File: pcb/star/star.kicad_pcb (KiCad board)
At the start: 2 copper layers, 58.9 x 56 mm, 24 parts, among them J1 POWER, U1 ESP-12F, U2 AP2112K-3.3

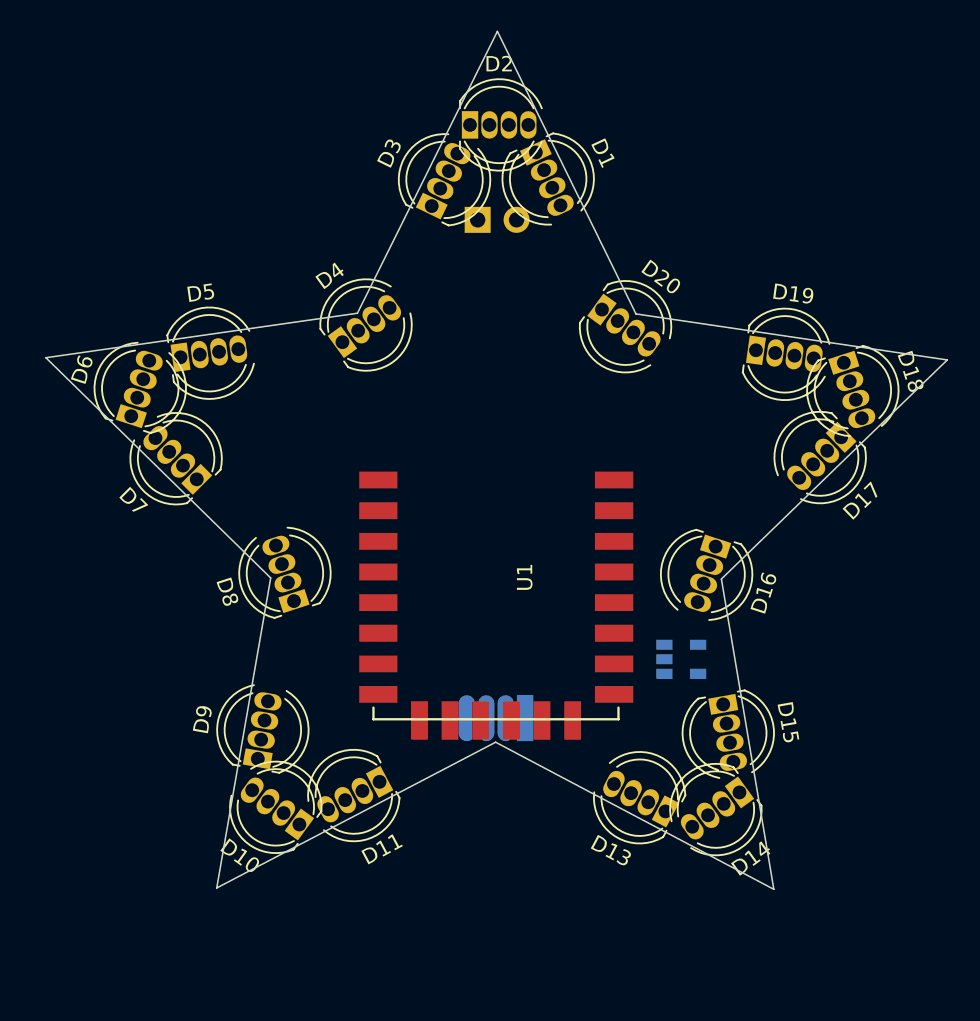
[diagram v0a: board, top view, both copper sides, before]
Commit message: layout first pass done
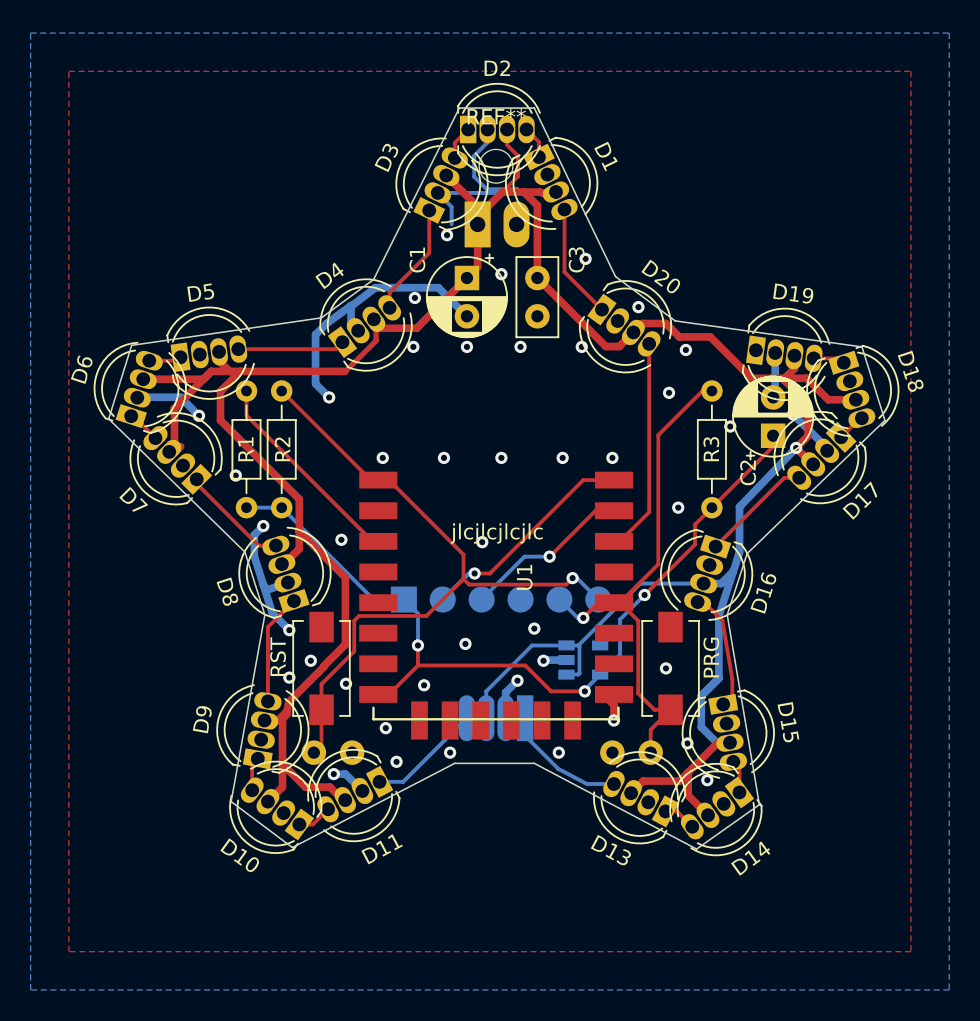
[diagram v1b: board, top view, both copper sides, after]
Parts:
- added C1: 10uF, Capacitor_THT:CP_Radial_D5.0mm_P2.50mm, F.Cu at (96.0, 71.0)
- added C2: 1uF, Capacitor_THT:CP_Radial_D5.0mm_P2.50mm, F.Cu at (116.0, 81.3)
- added C3: 100nF, Capacitor_THT:C_Disc_D5.0mm_W2.5mm_P2.50mm, F.Cu at (100.6, 71.0)
- added C4: 100nF, Capacitor_THT:C_Disc_D5.0mm_W2.5mm_P2.50mm, B.Cu at (88.5, 102.0)
- added C5: 100nF, Capacitor_THT:C_Disc_D5.0mm_W2.5mm_P2.50mm, B.Cu at (105.5, 102.0)
- added J2: Conn_01x06_Male, star:conn_01x06_SMD, B.Cu at (98.2, 92.0)
- added R1: 10k, Resistor_THT:R_Axial_DIN0204_L3.6mm_D1.6mm_P7.62mm_Horizontal, F.Cu at (81.6, 86.0)
- added R2: 10k, Resistor_THT:R_Axial_DIN0204_L3.6mm_D1.6mm_P7.62mm_Horizontal, F.Cu at (83.9, 86.0)
- added R3: 10k, Resistor_THT:R_Axial_DIN0204_L3.6mm_D1.6mm_P7.62mm_Horizontal, F.Cu at (112.0, 86.0)
- added REF**: MountingHole_2.2mm_M2, MountingHole:MountingHole_2.2mm_M2, F.Cu at (97.9, 63.7)
- added SW1: RST, Button_Switch_SMD:SW_SPST_EVQPE1, F.Cu at (86.5, 96.5)
- added SW2: PRG, Button_Switch_SMD:SW_SPST_EVQPE1, F.Cu at (109.3, 96.5)
- moved U2 6.40 mm to (103.6, 96.0)
- moved D1 0.36 mm to (100.7, 63.1), turned to 296 degrees
- moved D3 0.33 mm to (93.5, 66.6)
- moved D2 0.32 mm to (96.1, 61.3)
- moved J1 0.30 mm to (96.7, 67.5)
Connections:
- net Net-(U1-Pad2) renamed /ADC
- D20 pad 1: Net-(D20-Pad1) -> Net-(D1-Pad4)
- D20 pad 4: Net-(D19-Pad1) -> /LED_Din
- U1 pad 1: Net-(U1-Pad1) -> /RST
- U1 pad 12: Net-(U1-Pad12) -> /GPIO0
- U1 pad 14: Net-(U1-Pad14) -> /LED_Din
- U1 pad 15: Net-(U1-Pad15) -> /RXD
- U1 pad 16: Net-(U1-Pad16) -> /TXD
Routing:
- net +5V: track 0.00 -> 197.9 mm, vias 0 -> 1
- net GND: track 0.00 -> 62.0 mm, vias 0 -> 43
- net +3V3: track 0.00 -> 53.7 mm, vias 0 -> 3
- net /RST: track 0.00 -> 45.6 mm, vias 0 -> 1
- net /GPIO0: track 0.00 -> 34.0 mm, vias 0 -> 1
- net /LED_Din: track 0.00 -> 14.8 mm
- net Net-(R1-Pad2): track 0.00 -> 14.3 mm
- net /TXD: track 0.00 -> 13.7 mm, vias 0 -> 1
- net /RXD: track 0.00 -> 10.4 mm, vias 0 -> 1
- net Net-(D12-Pad1): track 0.00 -> 8.09 mm
- net /DoD15: track 0.00 -> 7.89 mm
- net Net-(D1-Pad4): track 0.00 -> 7.55 mm
- net Net-(D3-Pad1): track 0.00 -> 7.44 mm
- net Net-(D11-Pad1): track 0.00 -> 7.42 mm
- net Net-(D16-Pad1): track 0.00 -> 7.32 mm
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- added copper zone on B.Cu, net GND
- added copper zone on F.Cu, net GND
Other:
- board size 58.9 x 56 mm -> 50.7 x 48.4 mm
- board text added: "3V3"
- board text added: "5V"
- board text added: "GND"
- board text added: "IO0"
- board text added: "RST"
- board text added: "RXD"
- board text added: "TXD"
- board text added: "jlcjlcjlcjlc"
